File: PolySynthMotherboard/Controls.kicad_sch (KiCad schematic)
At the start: 97 parts, among them SW601 ENV1_B, SW602 ENV2_B, SW603 LFO1_B, SW604 LFO2_B, SW605 LFO3_B, SW606 MIX1_B, SW607 MIX2_B, SW608 ALT_B, SW609 FF_B, SW610 HP_B, SW611 HP_B, SW612 ENC_MENU, U204 ILI9341, U501 MCP23S17_SS

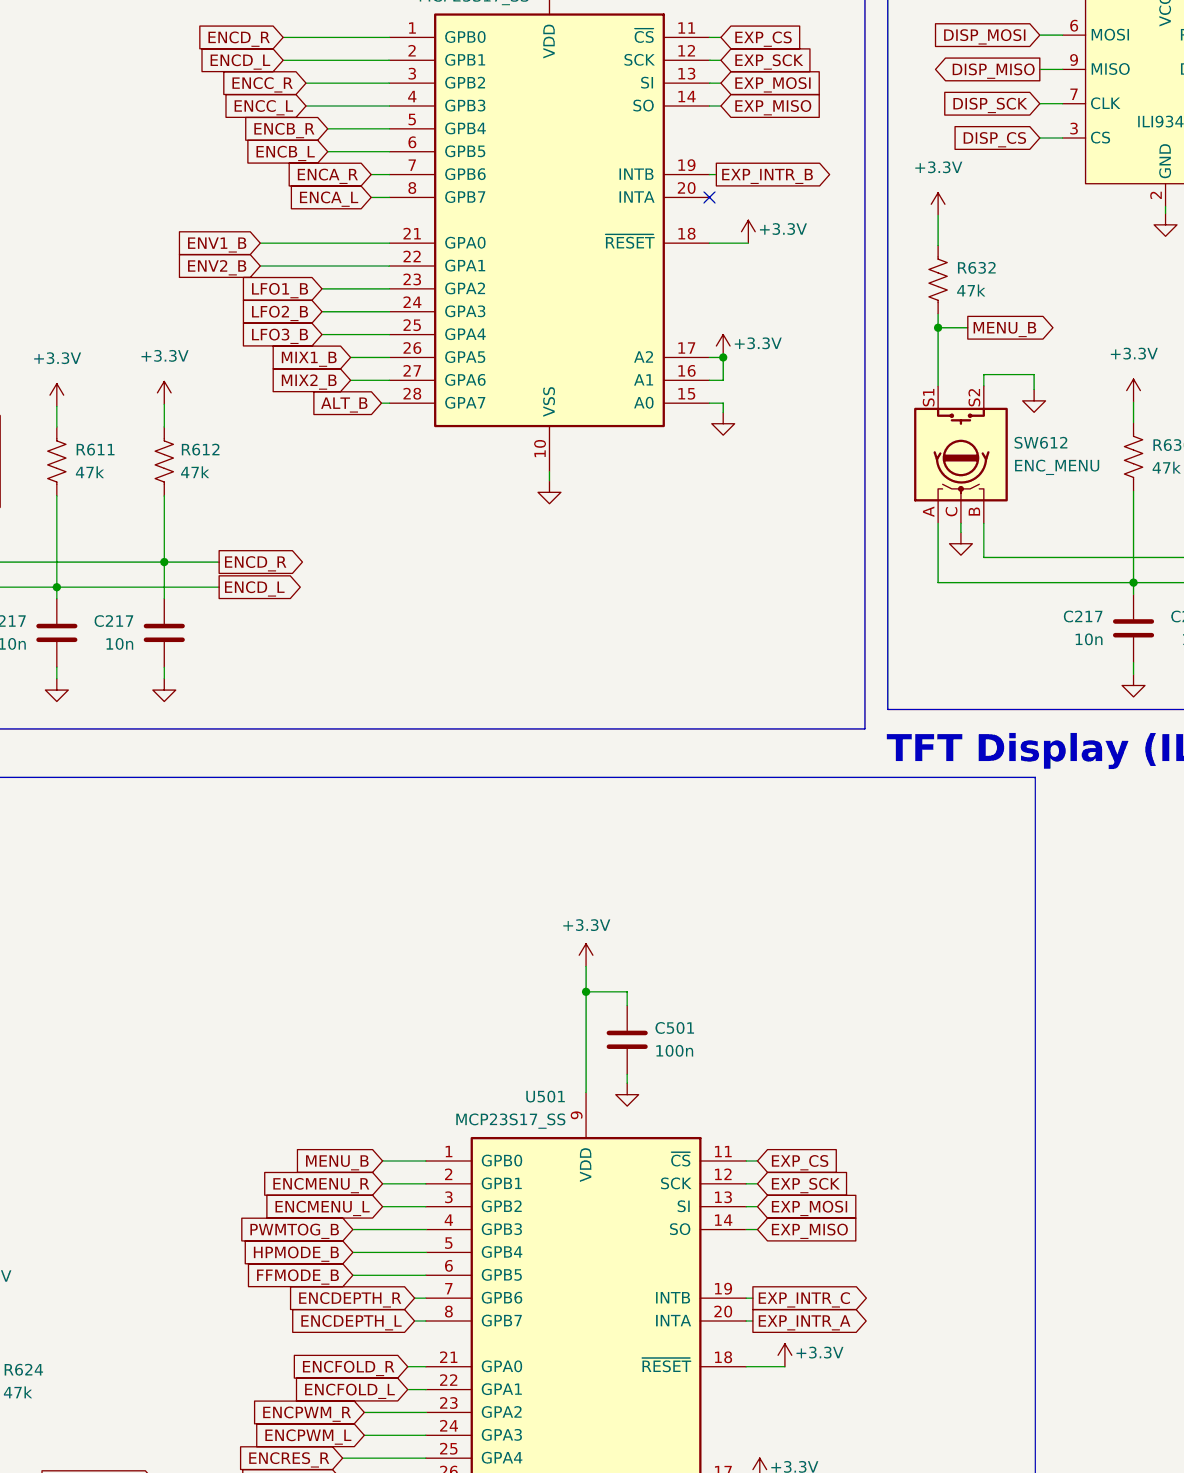
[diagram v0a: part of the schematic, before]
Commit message: motherboard rev1
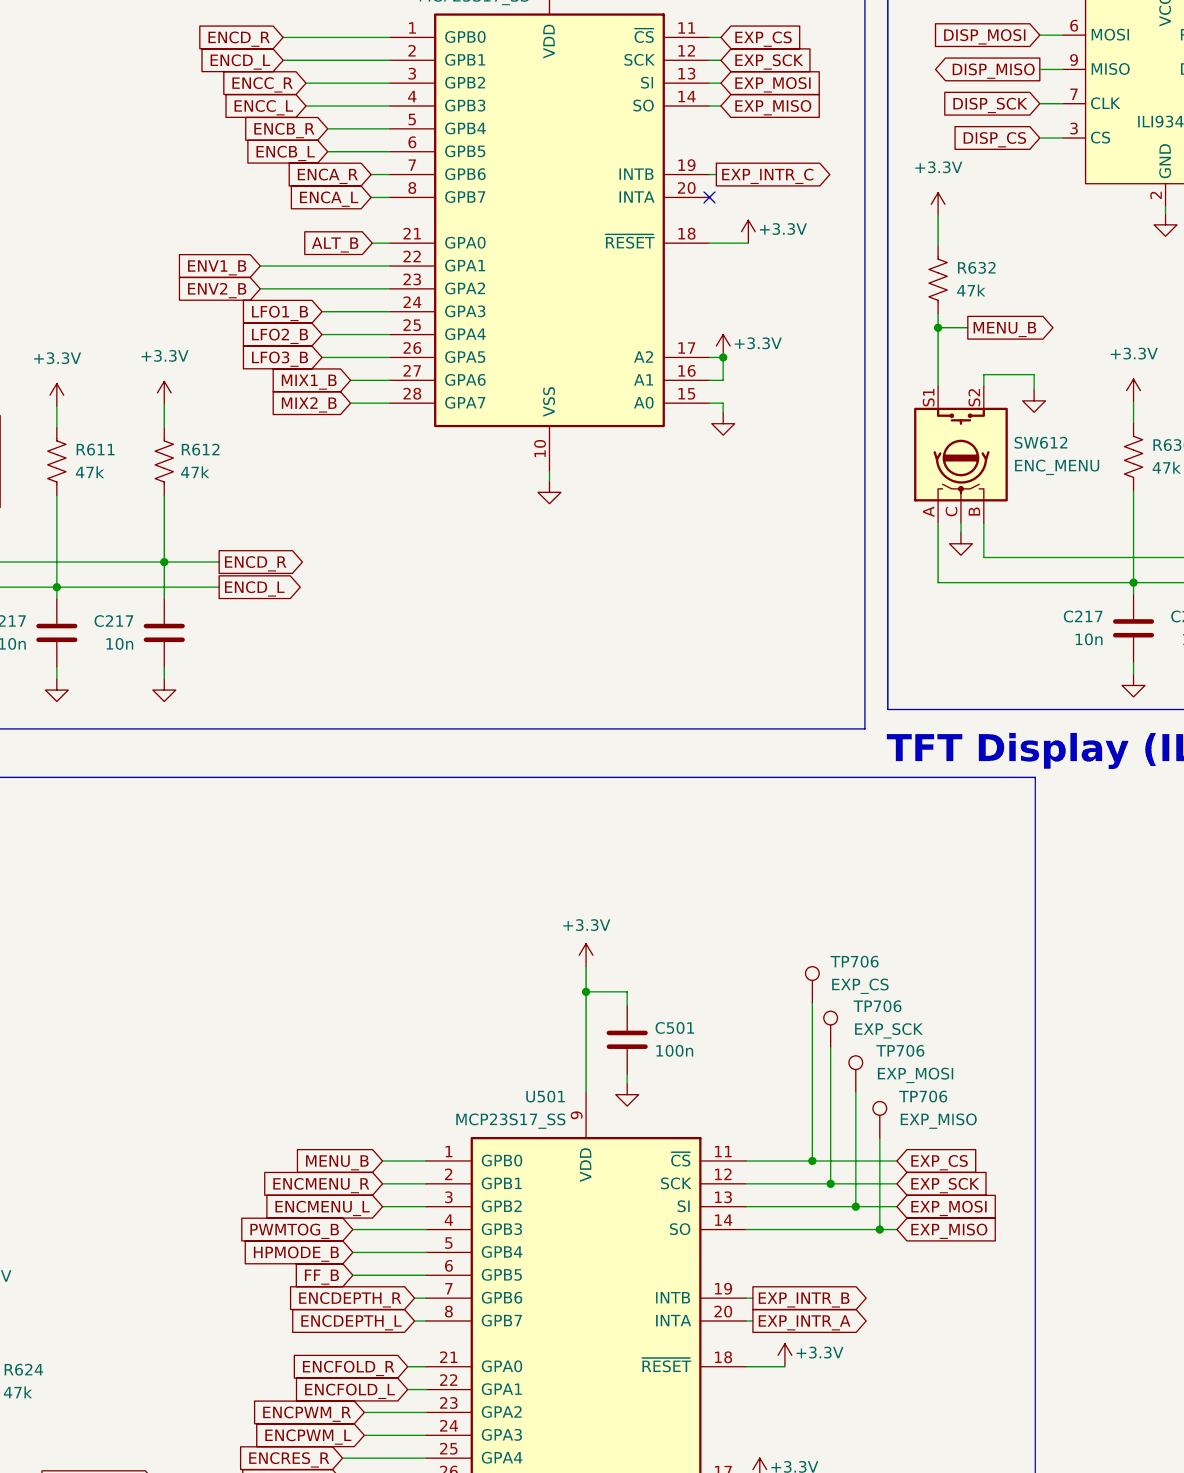
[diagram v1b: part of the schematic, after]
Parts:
- added TP706: EXP_SCK, TestPoint:TestPoint_Pad_D1.0mm_Value, symbol Connector:TestPoint
- added TP706: EXP_MISO, TestPoint:TestPoint_Pad_D1.0mm_Value, symbol Connector:TestPoint
- added TP706: EXP_MOSI, TestPoint:TestPoint_Pad_D1.0mm_Value, symbol Connector:TestPoint
- added TP706: EXP_CS, TestPoint:TestPoint_Pad_D1.0mm_Value, symbol Connector:TestPoint
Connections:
- net FFMODE_B is gone; now on net FF_B: U501.6 (GPB5)
- net ALT_B: now also U501.21 (GPA0); no longer U501.28 (GPA7)
- net ENV1_B: now also U501.22 (GPA1); no longer U501.21 (GPA0)
- net ENV2_B: now also U501.23 (GPA2); no longer U501.22 (GPA1)
- net EXP_CS: now also TP706.1
- net EXP_INTR_B: now also U501.19 (INTB); no longer U501.19 (INTB)
- net EXP_INTR_C: now also U501.19 (INTB); no longer U501.19 (INTB)
- net EXP_MISO: now also TP706.1
- net EXP_MOSI: now also TP706.1
- net EXP_SCK: now also TP706.1
- net LFO1_B: now also U501.24 (GPA3); no longer U501.23 (GPA2)
- net LFO2_B: now also U501.25 (GPA4); no longer U501.24 (GPA3)
- net LFO3_B: now also U501.26 (GPA5); no longer U501.25 (GPA4)
- net MIX1_B: now also U501.27 (GPA6); no longer U501.26 (GPA5)
- net MIX2_B: now also U501.28 (GPA7); no longer U501.27 (GPA6)
